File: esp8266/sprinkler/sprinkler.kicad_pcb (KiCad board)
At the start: 4 copper layers, 100.5 x 58.5 mm, 88 parts, among them J1 Terminal Block 1729128, J2 Terminal Block 1729128, J3 DF9B-19P-1V32, J4 Terminal Block 1729128, J5 Terminal Block 1729128, J6 Terminal Block 1729128, Q1 AO4407A, Q2 2N7002, Q3 2N7002, Q4 AON7401, Q5 2N7002, Q6 MMBT2222A, Q7 MMBT2222A, Q8 MMBT2222A, U1 MAX1873TEEE, U3 PC817, U4 LM2577S-ADJ_NOPB, U5 PCF8563T, U6 MMBT2907A-7-F, U7 MMBT2907A-7-F, U8 MMBT2907A-7-F, X1 DST310S

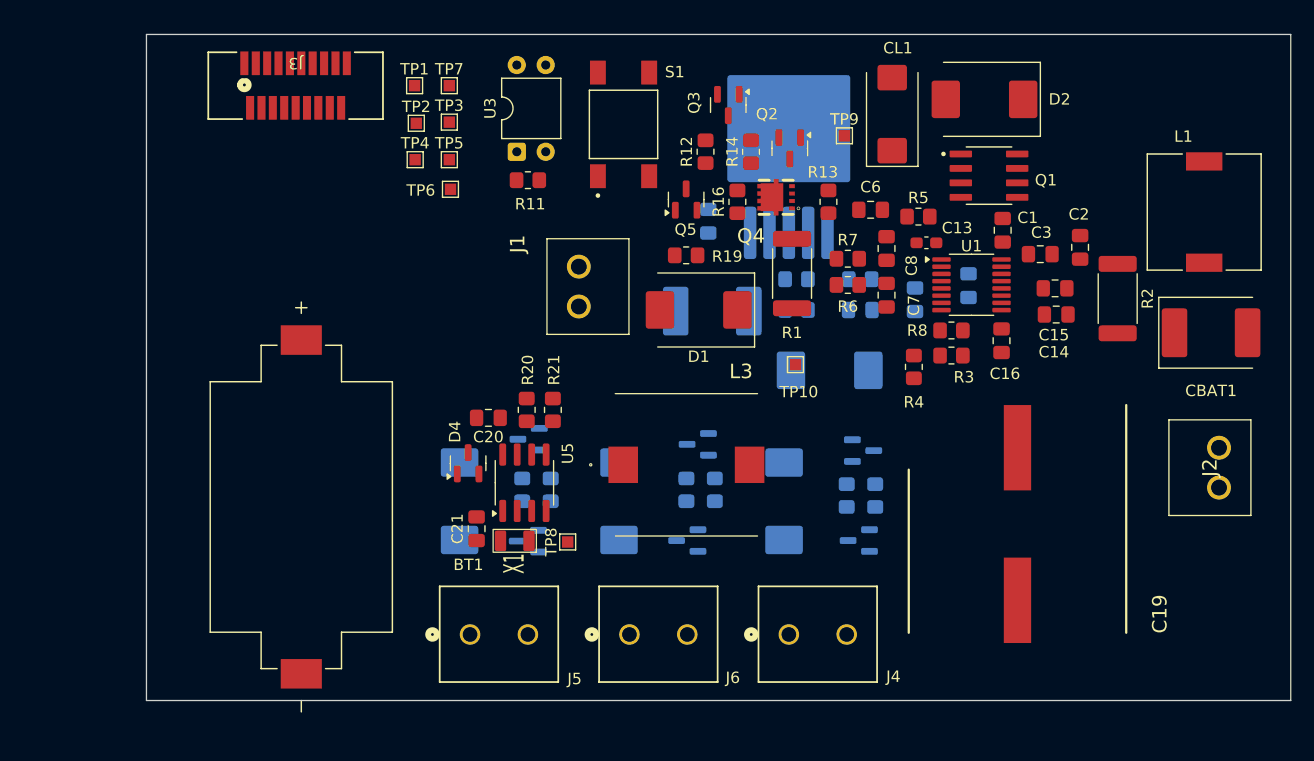
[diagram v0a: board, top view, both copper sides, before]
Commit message: Traces
Layout traces for the PCB
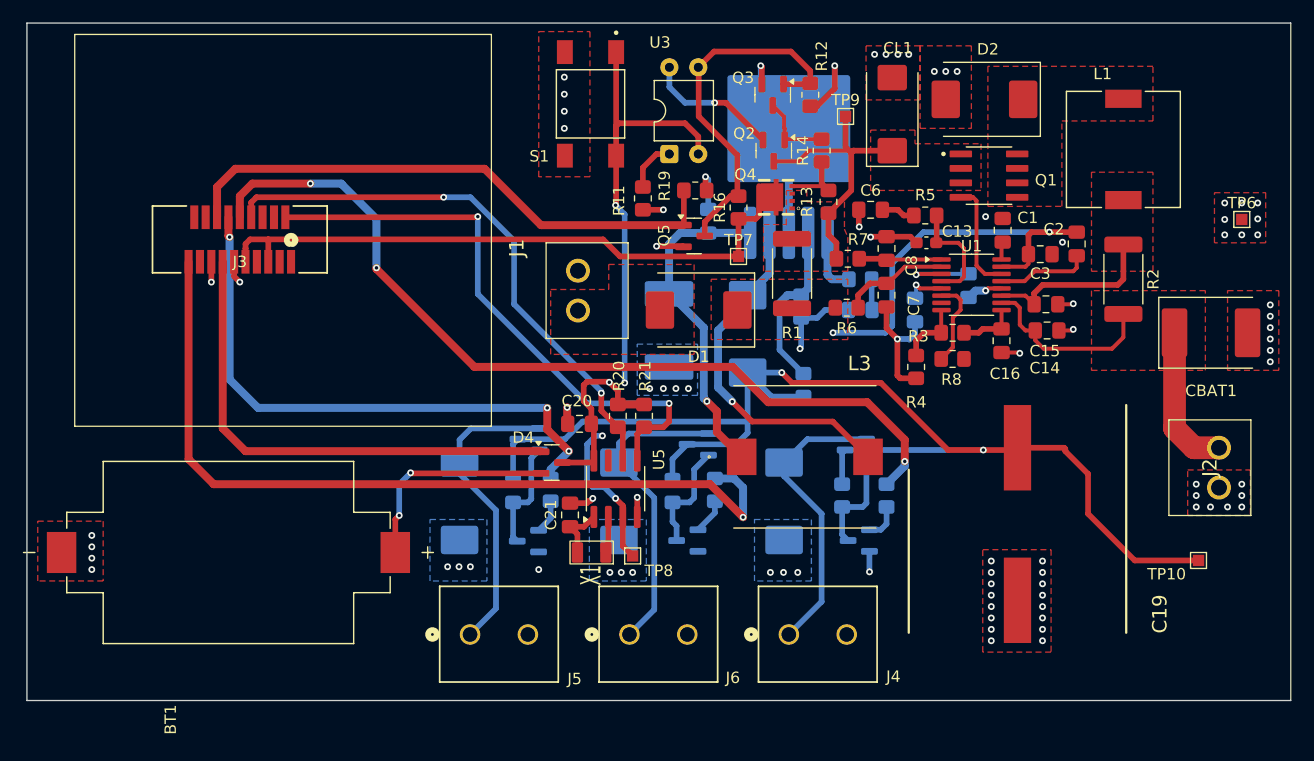
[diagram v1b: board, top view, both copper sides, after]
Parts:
- removed TP1, TP2, TP3, TP4, TP5: TestPoint, TestPoint:TestPoint_Pad_1.0x1.0mm
- moved TP6 69.6 mm to (192.0, 85.2)
- moved TP10 39.4 mm to (188.2, 115.2)
- moved TP7 29.5 mm to (147.8, 88.5)
- moved J3 14.4 mm to (104.0, 87.0), turned to 0 degrees
- moved U3 13.4 mm to (141.7, 79.5)
- moved R12 10.5 mm to (154.1, 74.3), turned to -90 degrees
- moved L3 10.4 mm to (153.6, 106.1)
- moved R11 10.2 mm to (139.4, 83.4), turned to 90 degrees
- moved L1 8.98 mm to (181.6, 79.1)
- moved C21 8.29 mm to (133.0, 111.2)
- moved C20 8.02 mm to (133.8, 103.2)
- moved R20 8.02 mm to (137.2, 102.5)
- moved R21 8.02 mm to (139.5, 102.5)
- moved U5 8.02 mm to (137.0, 108.9)
- moved D5 7.88 mm to (148.6, 95.3), turned to 90 degrees
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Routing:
- net +12V: track 0.00 -> 109.3 mm, vias 0 -> 2
- net GND: track 0.00 -> 78.4 mm, vias 0 -> 87
- net /Microcontroller/IO12: track 0.00 -> 77.3 mm, vias 0 -> 3
- net /Microcontroller/IO14: track 0.00 -> 73.6 mm, vias 0 -> 1
- net /Power Sheet/~{Int}: track 0.00 -> 59.0 mm, vias 0 -> 4
- net /Microcontroller/PowerIn: track 0.00 -> 55.4 mm
- net /Microcontroller/SDA: track 0.00 -> 51.7 mm, vias 0 -> 2
- net /Microcontroller/IO13: track 0.00 -> 50.9 mm, vias 0 -> 3
- net /Microcontroller/SCL: track 0.00 -> 49.4 mm, vias 0 -> 2
- net /Microcontroller/SwitchOff: track 0.00 -> 49.4 mm
- net /Microcontroller/esp8266_3V3: track 0.00 -> 43.4 mm
- net /Power Sheet/3V3: track 0.00 -> 35.7 mm, vias 0 -> 2
- net Net-(D1-K): track 0.00 -> 35.2 mm, vias 0 -> 2
- net Net-(Q3-G): track 0.00 -> 32.0 mm
- net Net-(D5-A): track 0.00 -> 31.1 mm, vias 0 -> 1
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- added copper zone on F.Cu, net /Power Sheet/SolarPower
- added copper zone on F.Cu, net /Power Sheet/SysLoad
- added copper zone on B.Cu, net GND
- added copper zone on F.Cu, net GND
- added copper zone on In1.Cu, net GND
- added copper zone on F.Cu, net Net-(D1-K)
- added copper zone on F.Cu, net Net-(D2-K)
- added copper zone on F.Cu, net Net-(U1-BATT)
- added copper zone on F.Cu, net Net-(U1-CSB)
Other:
- board size 100.5 x 58.5 mm -> 111 x 59.5 mm
